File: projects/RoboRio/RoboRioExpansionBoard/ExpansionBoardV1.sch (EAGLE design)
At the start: 91 parts, among them IC1 MC1525TO, Q1 5MHz

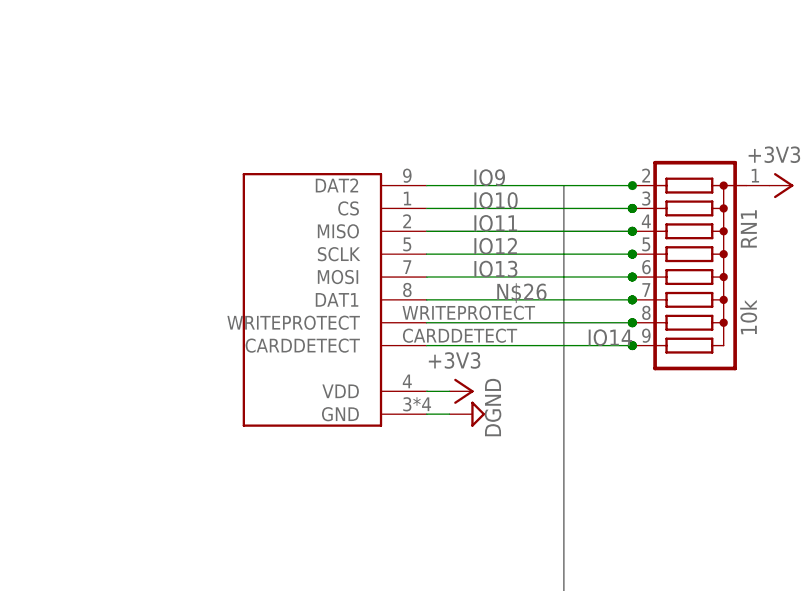
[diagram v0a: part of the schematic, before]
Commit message: Fixed SD card hotspot
Dubstep is very good music.
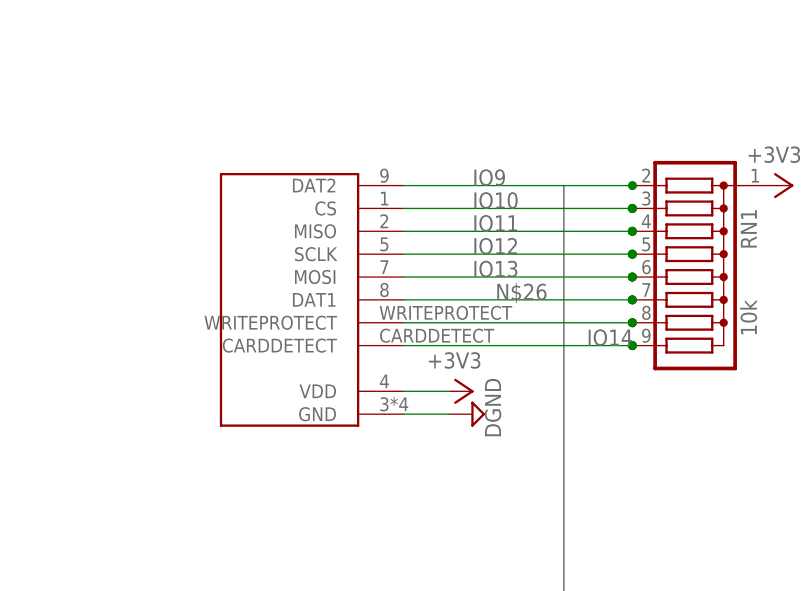
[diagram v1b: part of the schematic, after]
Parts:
- removed U$6: SDCARDLIBDEV, SDcardlibraryroborio:SDCARDLIBDEV
- added U$2: SDCARDLIBDEV, SDcardlibraryroborio:SDCARDLIBDEV
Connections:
- net +3V3: now also U$2.VDD; no longer U$6.VDD
- net DGND: now also U$2.GND; no longer U$6.GND
- net IO10: now also U$2.CS; no longer U$6.CS
- net IO11: now also U$2.MISO; no longer U$6.MISO
- net IO12: now also U$2.SCLK; no longer U$6.SCLK
- net IO13: now also U$2.MOSI; no longer U$6.MOSI
- net IO14: now also U$2.CARDDETECT; no longer U$6.CARDDETECT
- net IO9: now also U$2.DAT2; no longer U$6.DAT2
- net N$26: now also U$2.DAT1; no longer U$6.DAT1
- net N$27: now also U$2.WRITEPROTECT; no longer U$6.WRITEPROTECT
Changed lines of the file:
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@@
 <part name="P+10" library="supply1" deviceset="+5V" device=""/>
 <part name="C1" library="capacitor-wima" deviceset="C" device="7.5/6" value=".1uF"/>
-<part name="U$6" library="SDcardlibraryroborio" deviceset="SDCARDLIBDEV" device=""/>
 <part name="+3V5" library="supply1" deviceset="+3V3" device=""/>
 <part name="RN1" library="resistor-sil" deviceset="G08R" device="" value="10k"/>
@@
 <part name="+3V21" library="supply1" deviceset="+3V3" device=""/>
 <part name="SUPPLY50" library="supply2" deviceset="DGND" device=""/>
+<part name="U$2" library="SDcardlibraryroborio" deviceset="SDCARDLIBDEV" device=""/>
 </parts>
 <sheets>
@@
 <instance part="P+10" gate="1" x="-201.93" y="95.25" rot="MR0"/>
 <instance part="C1" gate="G$1" x="-7.62" y="152.4" rot="R90"/>
-<instance part="U$6" gate="G$1" x="-133.35" y="40.64"/>
 <instance part="+3V5" gate="G$1" x="-127" y="45.72" rot="R270"/>
 <instance part="RN1" gate="G$1" x="-104.1654" y="58.42" rot="R270"/>
@@
 <instance part="+3V21" gate="G$1" x="139.7" y="7.62" rot="R90"/>
 <instance part="SUPPLY50" gate="G$1" x="139.7" y="10.16" rot="R270"/>
+<instance part="U$2" gate="G$1" x="-148.59" y="55.88"/>
 </instances>
 <busses>
@@
 </segment>
 <segment>
-<pinref part="U$6" gate="G$1" pin="VDD"/>
 <pinref part="+3V5" gate="G$1" pin="+3V3"/>
-<wire x1="-132.08" y1="45.72" x2="-129.54" y2="45.72" width="0.1524" layer="91"/>
+<wire x1="-134.62" y1="45.72" x2="-129.54" y2="45.72" width="0.1524" layer="91"/>
+<pinref part="U$2" gate="G$1" pin="VDD"/>
 </segment>
 <segment>
@@
 </segment>
 <segment>
-<pinref part="U$6" gate="G$1" pin="DAT2"/>
-<wire x1="-116.84" y1="68.58" x2="-132.08" y2="68.58" width="0.1524" layer="91"/>
+<wire x1="-116.84" y1="68.58" x2="-134.62" y2="68.58" width="0.1524" layer="91"/>
 <label x="-127" y="68.58" size="1.778" layer="95"/>
+<pinref part="U$2" gate="G$1" pin="DAT2"/>
 </segment>
 <segment>
@@
 </segment>
 <segment>
-<pinref part="U$6" gate="G$1" pin="CS"/>
-<wire x1="-132.08" y1="66.04" x2="-116.84" y2="66.04" width="0.1524" layer="91"/>
-<wire x1="-116.84" y1="66.04" x2="-109.2454" y2="66.04" width="0.1524" layer="91"/>
+<wire x1="-134.62" y1="66.04" x2="-109.2454" y2="66.04" width="0.1524" layer="91"/>
 <junction x="-109.22" y="66.04"/>
 <wire x1="-109.2454" y1="66.04" x2="-109.22" y2="66.04" width="0.1524" layer="91"/>
@@
 <junction x="-109.2454" y="66.04"/>
 <label x="-127" y="66.04" size="1.778" layer="95"/>
+<pinref part="U$2" gate="G$1" pin="CS"/>
 </segment>
 <segment>
@@
 </segment>
 <segment>
-<pinref part="U$6" gate="G$1" pin="MISO"/>
 <wire x1="-109.22" y1="63.5" x2="-109.2454" y2="63.5" width="0.1524" layer="91"/>
 <junction x="-109.22" y="63.5"/>
-<wire x1="-109.2454" y1="63.5" x2="-116.84" y2="63.5" width="0.1524" layer="91"/>
-<wire x1="-116.84" y1="63.5" x2="-132.08" y2="63.5" width="0.1524" layer="91"/>
+<wire x1="-109.2454" y1="63.5" x2="-134.62" y2="63.5" width="0.1524" layer="91"/>
 <pinref part="RN1" gate="G$1" pin="4"/>
 <junction x="-109.2454" y="63.5"/>
 <label x="-127" y="63.5" size="1.778" layer="95"/>
+<pinref part="U$2" gate="G$1" pin="MISO"/>
 </segment>
 <segment>
@@
 </segment>
 <segment>
-<pinref part="U$6" gate="G$1" pin="SCLK"/>
-<wire x1="-132.08" y1="60.96" x2="-116.84" y2="60.96" width="0.1524" layer="91"/>
-<wire x1="-116.84" y1="60.96" x2="-109.2454" y2="60.96" width="0.1524" layer="91"/>
+<wire x1="-134.62" y1="60.96" x2="-109.2454" y2="60.96" width="0.1524" layer="91"/>
 <junction x="-109.22" y="60.96"/>
 <wire x1="-109.2454" y1="60.96" x2="-109.22" y2="60.96" width="0.1524" layer="91"/>
@@
 <junction x="-109.2454" y="60.96"/>
 <label x="-127" y="60.96" size="1.778" layer="95"/>
+<pinref part="U$2" gate="G$1" pin="SCLK"/>
 </segment>
 </net>
@@
 </segment>
 <segment>
-<pinref part="U$6" gate="G$1" pin="MOSI"/>
 <wire x1="-109.22" y1="58.42" x2="-109.2454" y2="58.42" width="0.1524" layer="91"/>
 <junction x="-109.22" y="58.42"/>
-<wire x1="-109.2454" y1="58.42" x2="-116.84" y2="58.42" width="0.1524" layer="91"/>
-<wire x1="-116.84" y1="58.42" x2="-132.08" y2="58.42" width="0.1524" layer="91"/>
+<wire x1="-109.2454" y1="58.42" x2="-134.62" y2="58.42" width="0.1524" layer="91"/>
 <pinref part="RN1" gate="G$1" pin="6"/>
 <junction x="-109.2454" y="58.42"/>
 <label x="-127" y="58.42" size="1.778" layer="95"/>
+<pinref part="U$2" gate="G$1" pin="MOSI"/>
 </segment>
 </net>
@@
 </segment>
 <segment>
-<pinref part="U$6" gate="G$1" pin="CARDDETECT"/>
-<wire x1="-132.08" y1="50.8" x2="-116.84" y2="50.8" width="0.1524" layer="91"/>
-<wire x1="-116.84" y1="50.8" x2="-109.2454" y2="50.8" width="0.1524" layer="91"/>
+<wire x1="-134.62" y1="50.8" x2="-109.2454" y2="50.8" width="0.1524" layer="91"/>
 <junction x="-109.22" y="50.8"/>
 <wire x1="-109.2454" y1="50.8" x2="-109.22" y2="50.8" width="0.1524" layer="91"/>
@@
 <junction x="-109.2454" y="50.8"/>
 <label x="-114.3" y="50.8" size="1.778" layer="95"/>
+<pinref part="U$2" gate="G$1" pin="CARDDETECT"/>
 </segment>
 <segment>
@@
 <net name="N$26" class="0">
 <segment>
-<pinref part="U$6" gate="G$1" pin="DAT1"/>
-<wire x1="-132.08" y1="55.88" x2="-116.84" y2="55.88" width="0.1524" layer="91"/>
-<wire x1="-116.84" y1="55.88" x2="-109.2454" y2="55.88" width="0.1524" layer="91"/>
+<wire x1="-134.62" y1="55.88" x2="-109.2454" y2="55.88" width="0.1524" layer="91"/>
 <junction x="-109.22" y="55.88"/>
 <pinref part="RN1" gate="G$1" pin="7"/>
@@
 <junction x="-109.2454" y="55.88"/>
 <label x="-124.46" y="55.88" size="1.778" layer="95"/>
+<pinref part="U$2" gate="G$1" pin="DAT1"/>
 </segment>
 </net>
 <net name="N$27" class="0">
 <segment>
-<pinref part="U$6" gate="G$1" pin="WRITEPROTECT"/>
 <wire x1="-109.22" y1="53.34" x2="-109.2454" y2="53.34" width="0.1524" layer="91"/>
 <junction x="-109.22" y="53.34"/>
 <pinref part="RN1" gate="G$1" pin="8"/>
-<wire x1="-109.2454" y1="53.34" x2="-116.84" y2="53.34" width="0.1524" layer="91"/>
-<wire x1="-116.84" y1="53.34" x2="-132.08" y2="53.34" width="0.1524" layer="91"/>
+<wire x1="-109.2454" y1="53.34" x2="-134.62" y2="53.34" width="0.1524" layer="91"/>
 <junction x="-109.2454" y="53.34"/>
+<pinref part="U$2" gate="G$1" pin="WRITEPROTECT"/>
 </segment>
 </net>
@@
 </segment>
 <segment>
-<pinref part="U$6" gate="G$1" pin="GND"/>
 <pinref part="SUPPLY10" gate="G$1" pin="DGND"/>
-<wire x1="-132.08" y1="43.18" x2="-129.54" y2="43.18" width="0.1524" layer="91"/>
-</segment>
-<segment>
+<wire x1="-134.62" y1="43.18" x2="-129.54" y2="43.18" width="0.1524" layer="91"/>
+<pinref part="U$2" gate="G$1" pin="GND"/>
+</segment>
+<segment>
